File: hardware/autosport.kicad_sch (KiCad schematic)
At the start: 10 parts, among them J2 AS022-55SN

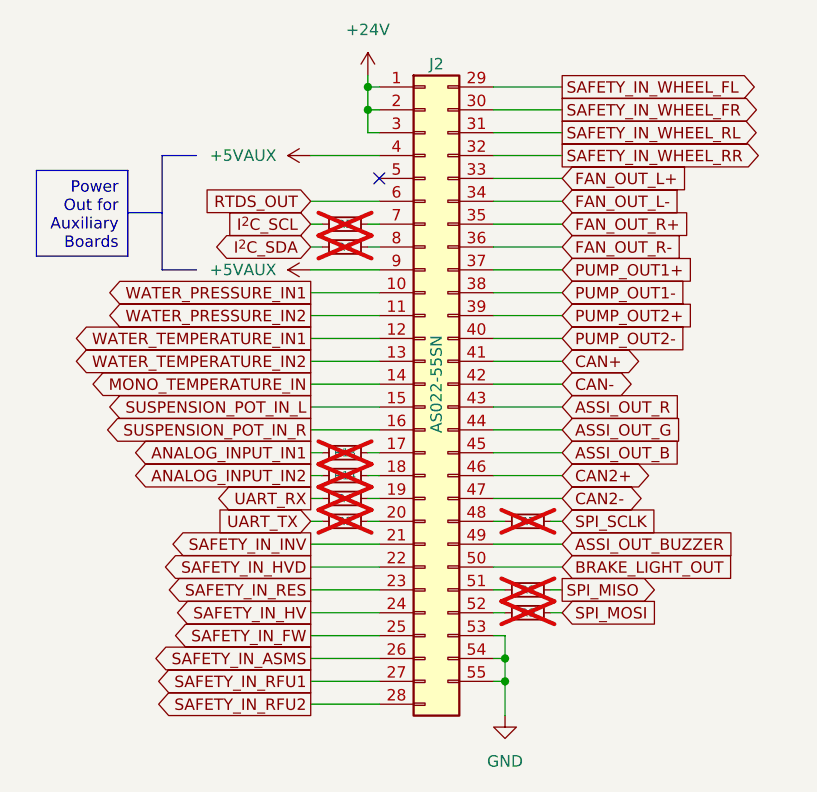
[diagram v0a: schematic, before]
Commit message: Use in-amps
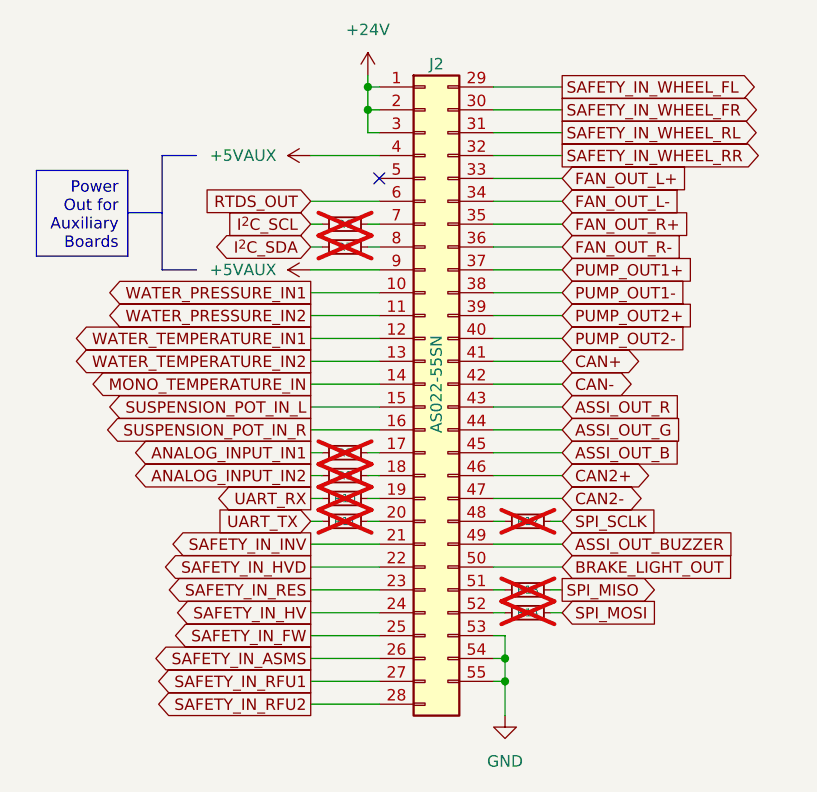
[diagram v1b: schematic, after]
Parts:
- renumbered R4 to R10, R3 to R11, R7 to R12, R8 to R13, R9 to R14, R5 to R6, R6 to R7, R13 to R8, R14 to R9
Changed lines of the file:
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@@
   (symbol (lib_id "Device:R_Small") (at 139.7 85.09 270) (mirror x) (unit 1)
     (in_bom yes) (on_board yes) (dnp yes)
-    (property "Reference" "R6" (at 139.7 85.09 90)
+    (property "Reference" "R7" (at 139.7 85.09 90)
       (effects (font (size 0.9 0.9)))
     )
@@
       (project "rearbox"
         (path "/b652b05a-4e3d-4ad1-b032-18886abe7d45/cf65c657-8245-46fb-8929-d241bd579513"
+          (reference "R7") (unit 1)
+        )
+        (path "/b652b05a-4e3d-4ad1-b032-18886abe7d45"
           (reference "R6") (unit 1)
         )
-        (path "/b652b05a-4e3d-4ad1-b032-18886abe7d45"
-          (reference "R6") (unit 1)
-        )
       )
     )
@@
   (symbol (lib_id "Device:R_Small") (at 160.02 123.19 90) (unit 1)
     (in_bom yes) (on_board yes) (dnp yes)
-    (property "Reference" "R8" (at 160.02 123.19 90)
+    (property "Reference" "R13" (at 160.02 123.19 90)
       (effects (font (size 0.9 0.9)))
     )
@@
       (project "rearbox"
         (path "/b652b05a-4e3d-4ad1-b032-18886abe7d45/cf65c657-8245-46fb-8929-d241bd579513"
-          (reference "R8") (unit 1)
+          (reference "R13") (unit 1)
         )
         (path "/b652b05a-4e3d-4ad1-b032-18886abe7d45"
@@
   (symbol (lib_id "Device:R_Small") (at 139.7 82.55 270) (mirror x) (unit 1)
     (in_bom yes) (on_board yes) (dnp yes)
-    (property "Reference" "R5" (at 139.7 82.55 90)
+    (property "Reference" "R6" (at 139.7 82.55 90)
       (effects (font (size 0.9 0.9)))
     )
@@
       (project "rearbox"
         (path "/b652b05a-4e3d-4ad1-b032-18886abe7d45/cf65c657-8245-46fb-8929-d241bd579513"
+          (reference "R6") (unit 1)
+        )
+        (path "/b652b05a-4e3d-4ad1-b032-18886abe7d45"
           (reference "R5") (unit 1)
         )
-        (path "/b652b05a-4e3d-4ad1-b032-18886abe7d45"
-          (reference "R5") (unit 1)
-        )
       )
     )
@@
   (symbol (lib_id "Device:R_Small") (at 160.02 115.57 90) (unit 1)
     (in_bom yes) (on_board yes) (dnp yes)
-    (property "Reference" "R7" (at 160.02 115.57 90)
+    (property "Reference" "R12" (at 160.02 115.57 90)
       (effects (font (size 0.9 0.9)))
     )
@@
       (project "rearbox"
         (path "/b652b05a-4e3d-4ad1-b032-18886abe7d45/cf65c657-8245-46fb-8929-d241bd579513"
-          (reference "R7") (unit 1)
+          (reference "R12") (unit 1)
         )
         (path "/b652b05a-4e3d-4ad1-b032-18886abe7d45"
@@
   (symbol (lib_id "Device:R_Small") (at 139.7 110.49 90) (unit 1)
     (in_bom yes) (on_board yes) (dnp yes)
-    (property "Reference" "R14" (at 139.7 110.49 90)
+    (property "Reference" "R9" (at 139.7 110.49 90)
       (effects (font (size 0.9 0.9)))
     )
@@
       (project "rearbox"
         (path "/b652b05a-4e3d-4ad1-b032-18886abe7d45/cf65c657-8245-46fb-8929-d241bd579513"
-          (reference "R14") (unit 1)
+          (reference "R9") (unit 1)
         )
       )
@@
   (symbol (lib_id "Device:R_Small") (at 139.7 115.57 270) (unit 1)
     (in_bom yes) (on_board yes) (dnp yes)
-    (property "Reference" "R3" (at 139.7 115.57 90)
+    (property "Reference" "R11" (at 139.7 115.57 90)
       (effects (font (size 0.9 0.9)))
     )
@@
       (project "rearbox"
         (path "/b652b05a-4e3d-4ad1-b032-18886abe7d45/cf65c657-8245-46fb-8929-d241bd579513"
-          (reference "R3") (unit 1)
+          (reference "R11") (unit 1)
         )
         (path "/b652b05a-4e3d-4ad1-b032-18886abe7d45"
@@
   (symbol (lib_id "Device:R_Small") (at 139.7 107.95 90) (unit 1)
     (in_bom yes) (on_board yes) (dnp yes)
-    (property "Reference" "R13" (at 139.7 107.95 90)
+    (property "Reference" "R8" (at 139.7 107.95 90)
       (effects (font (size 0.9 0.9)))
     )
@@
       (project "rearbox"
         (path "/b652b05a-4e3d-4ad1-b032-18886abe7d45/cf65c657-8245-46fb-8929-d241bd579513"
-          (reference "R13") (unit 1)
+          (reference "R8") (unit 1)
         )
       )
@@
   (symbol (lib_id "Device:R_Small") (at 160.02 125.73 90) (unit 1)
     (in_bom yes) (on_board yes) (dnp yes)
-    (property "Reference" "R9" (at 160.02 125.73 90)
+    (property "Reference" "R14" (at 160.02 125.73 90)
       (effects (font (size 0.9 0.9)))
     )
@@
       (project "rearbox"
         (path "/b652b05a-4e3d-4ad1-b032-18886abe7d45/cf65c657-8245-46fb-8929-d241bd579513"
+          (reference "R14") (unit 1)
+        )
+        (path "/b652b05a-4e3d-4ad1-b032-18886abe7d45"
           (reference "R9") (unit 1)
         )
-        (path "/b652b05a-4e3d-4ad1-b032-18886abe7d45"
-          (reference "R9") (unit 1)
-        )
       )
     )
@@
   (symbol (lib_id "Device:R_Small") (at 139.7 113.03 270) (unit 1)
     (in_bom yes) (on_board yes) (dnp yes)
-    (property "Reference" "R4" (at 139.7 113.03 90)
+    (property "Reference" "R10" (at 139.7 113.03 90)
       (effects (font (size 0.9 0.9)))
     )
@@
       (project "rearbox"
         (path "/b652b05a-4e3d-4ad1-b032-18886abe7d45/cf65c657-8245-46fb-8929-d241bd579513"
-          (reference "R4") (unit 1)
-        )
-        (path "/b652b05a-4e3d-4ad1-b032-18886abe7d45"
+          (reference "R10") (unit 1)
+        )
+        (path "/b652b05a-4e3d-4ad1-b032-18886abe7d45"
